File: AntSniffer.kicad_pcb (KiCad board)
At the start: 4 copper layers, 50.1 x 30.1 mm, 6 parts, among them CN1 X2026WRS-2X09D-LPSW, CN2 X2026WRS-2X09D-LPSW, J1 Conn_01x10_MountingPin

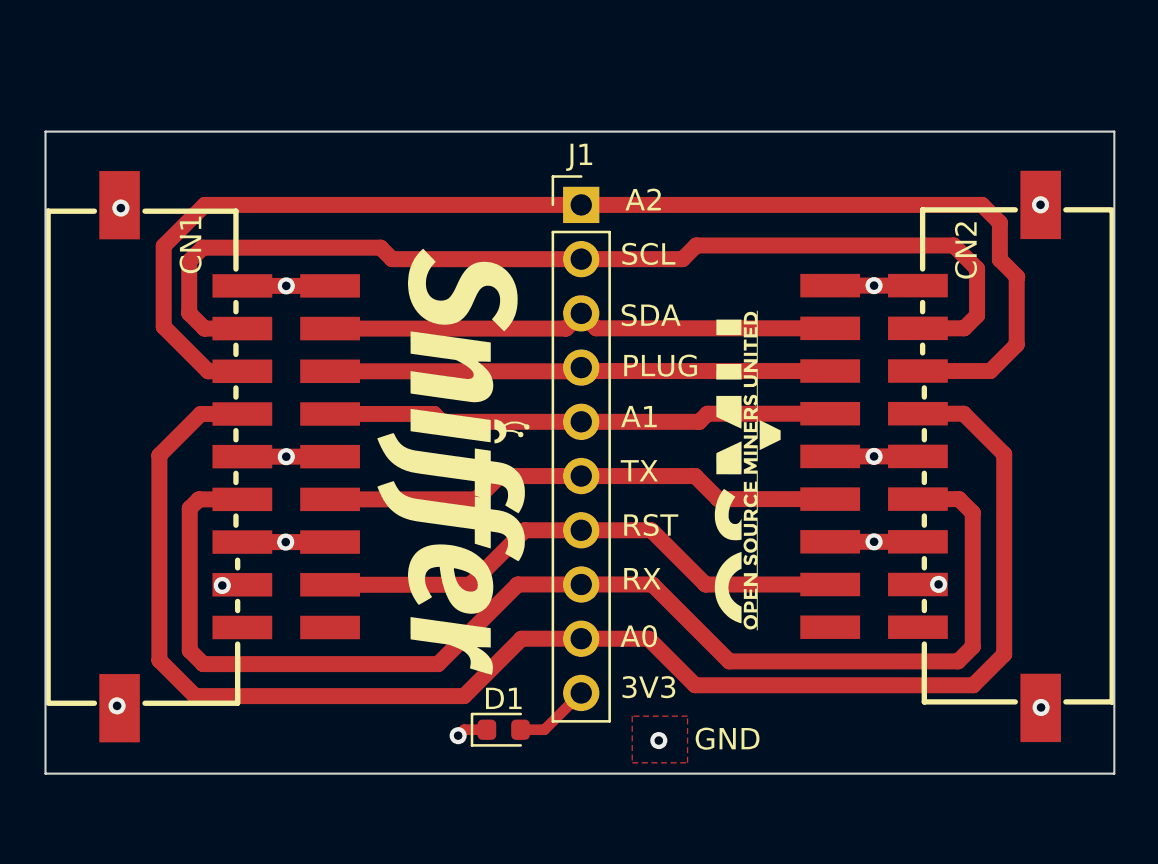
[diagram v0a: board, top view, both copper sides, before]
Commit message: Release V2.1
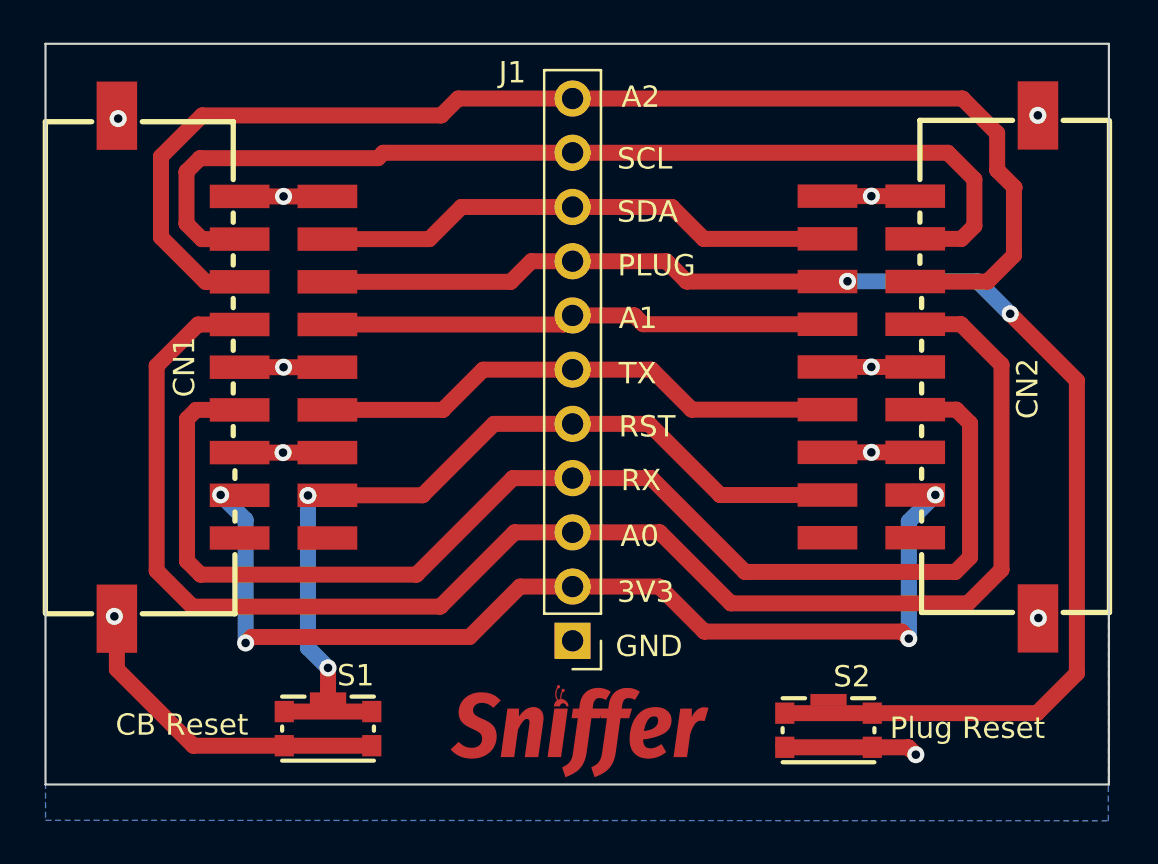
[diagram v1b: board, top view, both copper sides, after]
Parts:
- removed D1: LED, LED_SMD:LED_0603_1608Metric
- added S1: 435441019830, DOWNLOADED:435441019830, F.Cu at (156.7, 70.5)
- added S2: 435441019830, DOWNLOADED:435441019830, F.Cu at (180.2, 70.6)
- Ge: moved to B.Cu
- J1: value Conn_01x10_MountingPin -> Conn_01x11_Pin; footprint Connector_PinHeader_2.54mm:PinHeader_1x10_P2.54mm_Vertical -> Connector_PinHeader_2.54mm:PinHeader_1x11_P2.54mm_Vertical
- moved J1 20.4 mm to (168.2, 66.4), turned to 180 degrees
- moved Ge 14.7 mm to (168.6, 70.9), turned to 180 degrees
- moved G*** 13.9 mm to (168.5, 70.6), turned to 0 degrees
- moved CN1 4.19 mm to (151.8, 53.6)
- moved CN2 4.19 mm to (185.0, 53.6)
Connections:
- J1 pad 1: /A2 -> GND
- J1 pad 10: /3V3 -> /SCL
- J1 pad 2: /SCL -> /3V3
- J1 pad 3: /SDA -> /A0
- J1 pad 4: /PLUG -> /RX
- J1 pad 5: /A1 -> /RST
- J1 pad 7: /RST -> /A1
- J1 pad 8: /RX -> /PLUG
- J1 pad 9: /A0 -> /SDA
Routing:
- net /3V3: track 5.48 -> 49.8 mm, vias 2 -> 4
- net /PLUG: track 23.6 -> 65.1 mm, vias 0 -> 2
- net GND: track 26.5 -> 47.2 mm, vias 12 -> 11
- net /RST: track 25.6 -> 40.2 mm, vias 0 -> 2
- net /A0: track 71.4 -> 72.5 mm
- net /A2: track 59.8 -> 60.5 mm
- net /RX: track 58.7 -> 59.3 mm
- net /TX: track 24.3 -> 25.0 mm
- net /SDA: track 24.0 -> 24.7 mm
- added copper zone on B.Cu, net GND
- removed copper zone on In2.Cu, net /3V3
- removed copper zone on F.Cu, net GND
- removed copper zone on In1.Cu, net GND
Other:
- board size 50.1 x 30.1 mm -> 49.8 x 34.7 mm
- copper layers 4 -> 2
- board text added: "CB Reset"
- board text added: "Order Number"
- board text added: "Plug Reset"
- board text added: "Revision 2.1"
- board text removed: "Revision 1"
- board text removed: "The AntSniffer by OSMU"
